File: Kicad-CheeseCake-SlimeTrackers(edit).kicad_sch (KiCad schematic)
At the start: 24 parts, among them J2 USB_C-16p, Q1 UMH3N, SW1 SW_SPDT, U2 TP4057, U3 CH340K

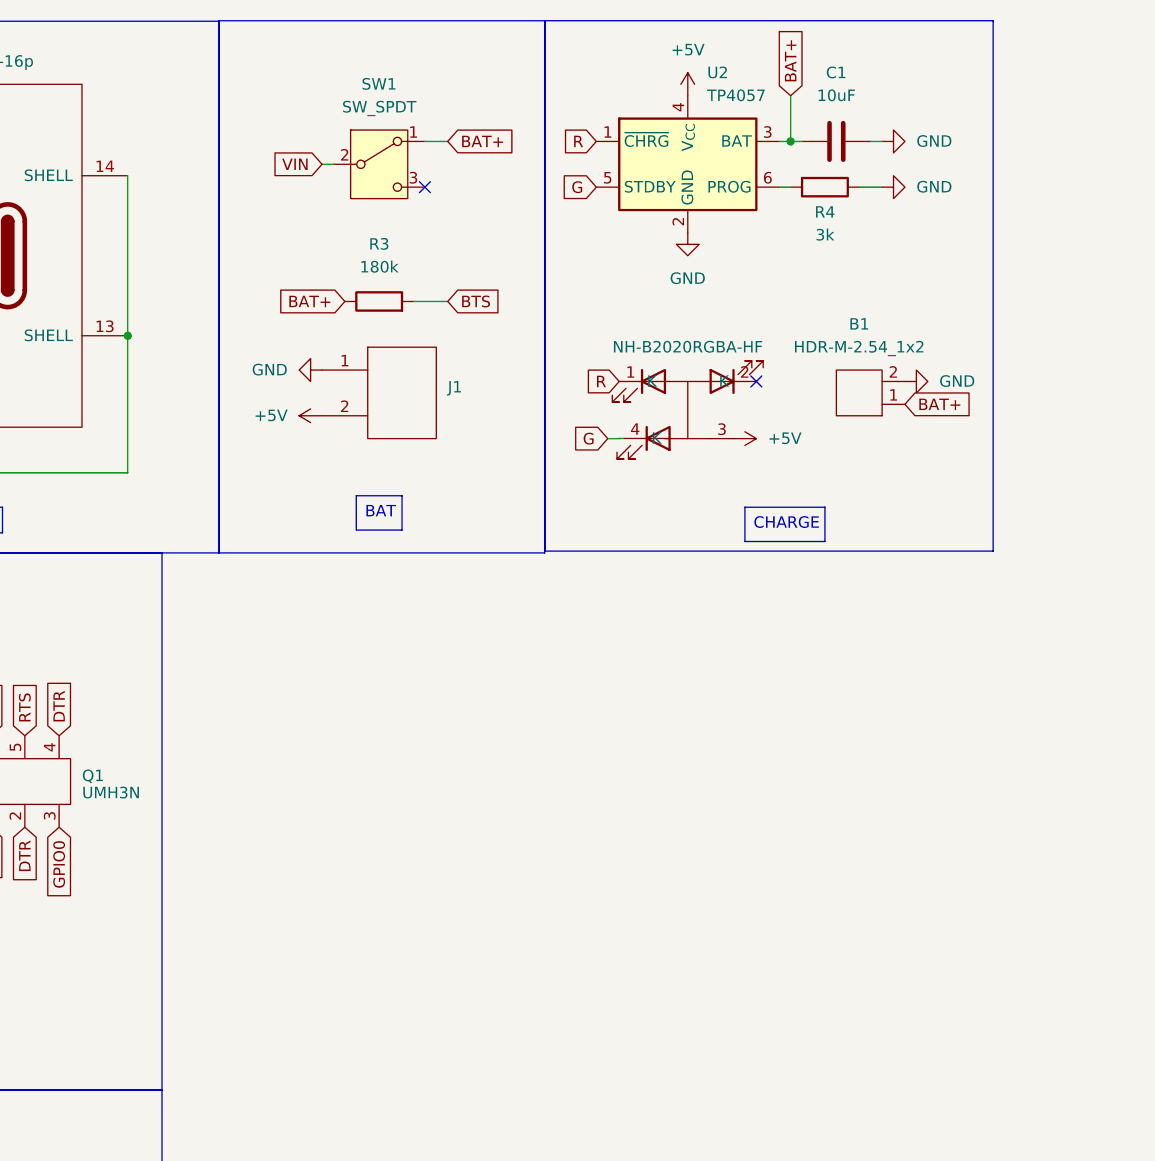
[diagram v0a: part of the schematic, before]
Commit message: updt
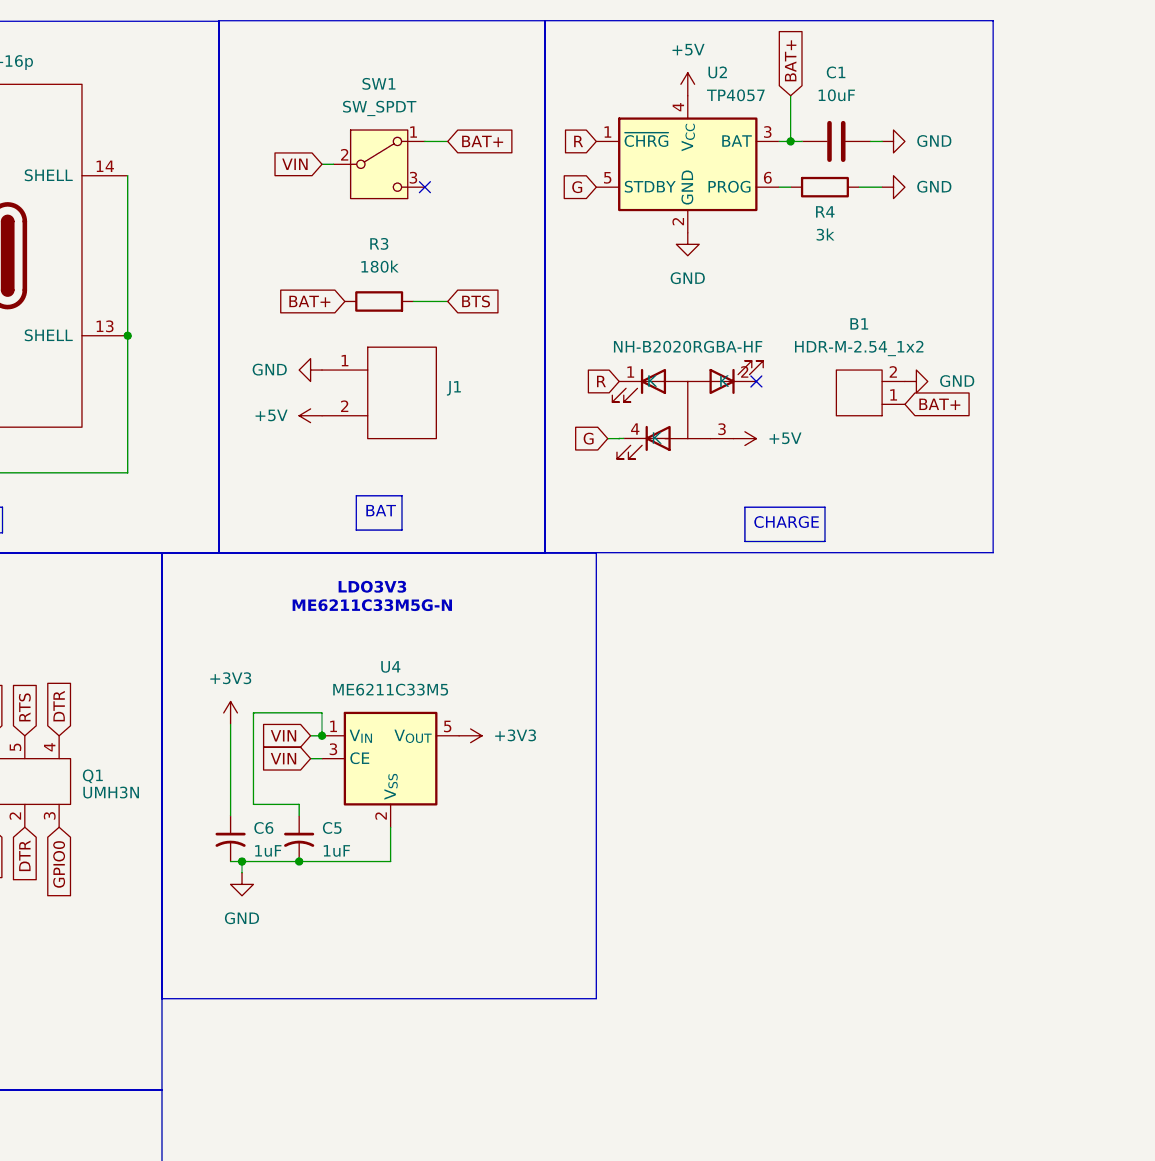
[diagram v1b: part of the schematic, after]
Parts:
- added C5, C6: 1uF, symbol Device:C_Small_US
- added U4: ME6211C33M5, Package_TO_SOT_SMD:SOT-23-5, symbol Regulator_Linear:ME6211C33M5
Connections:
- net +3V3: now also C6.1, U4.5 (V_{OUT})
- net GND: now also C5.2, C6.2, U4.2 (V_{SS})
- net VIN: now also C5.1, U4.1 (V_{IN}), U4.3 (CE)
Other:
- note added: "LDO3V3 ME6211C33M5G-N"

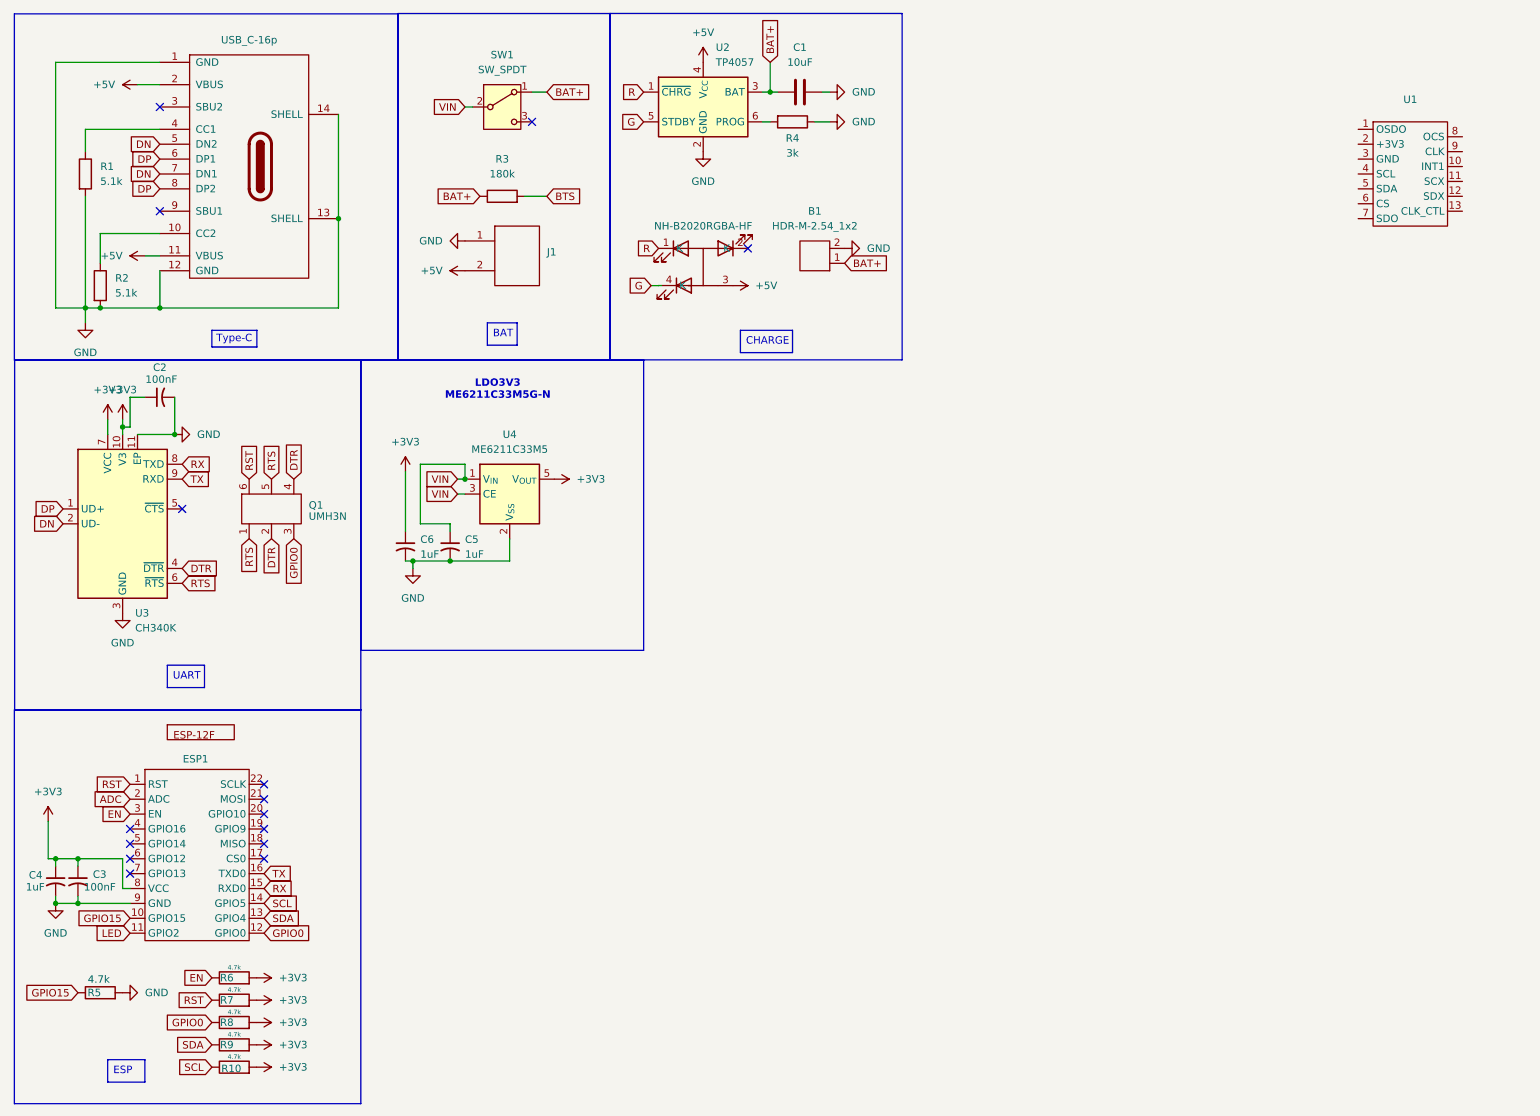
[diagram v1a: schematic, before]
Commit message: updt
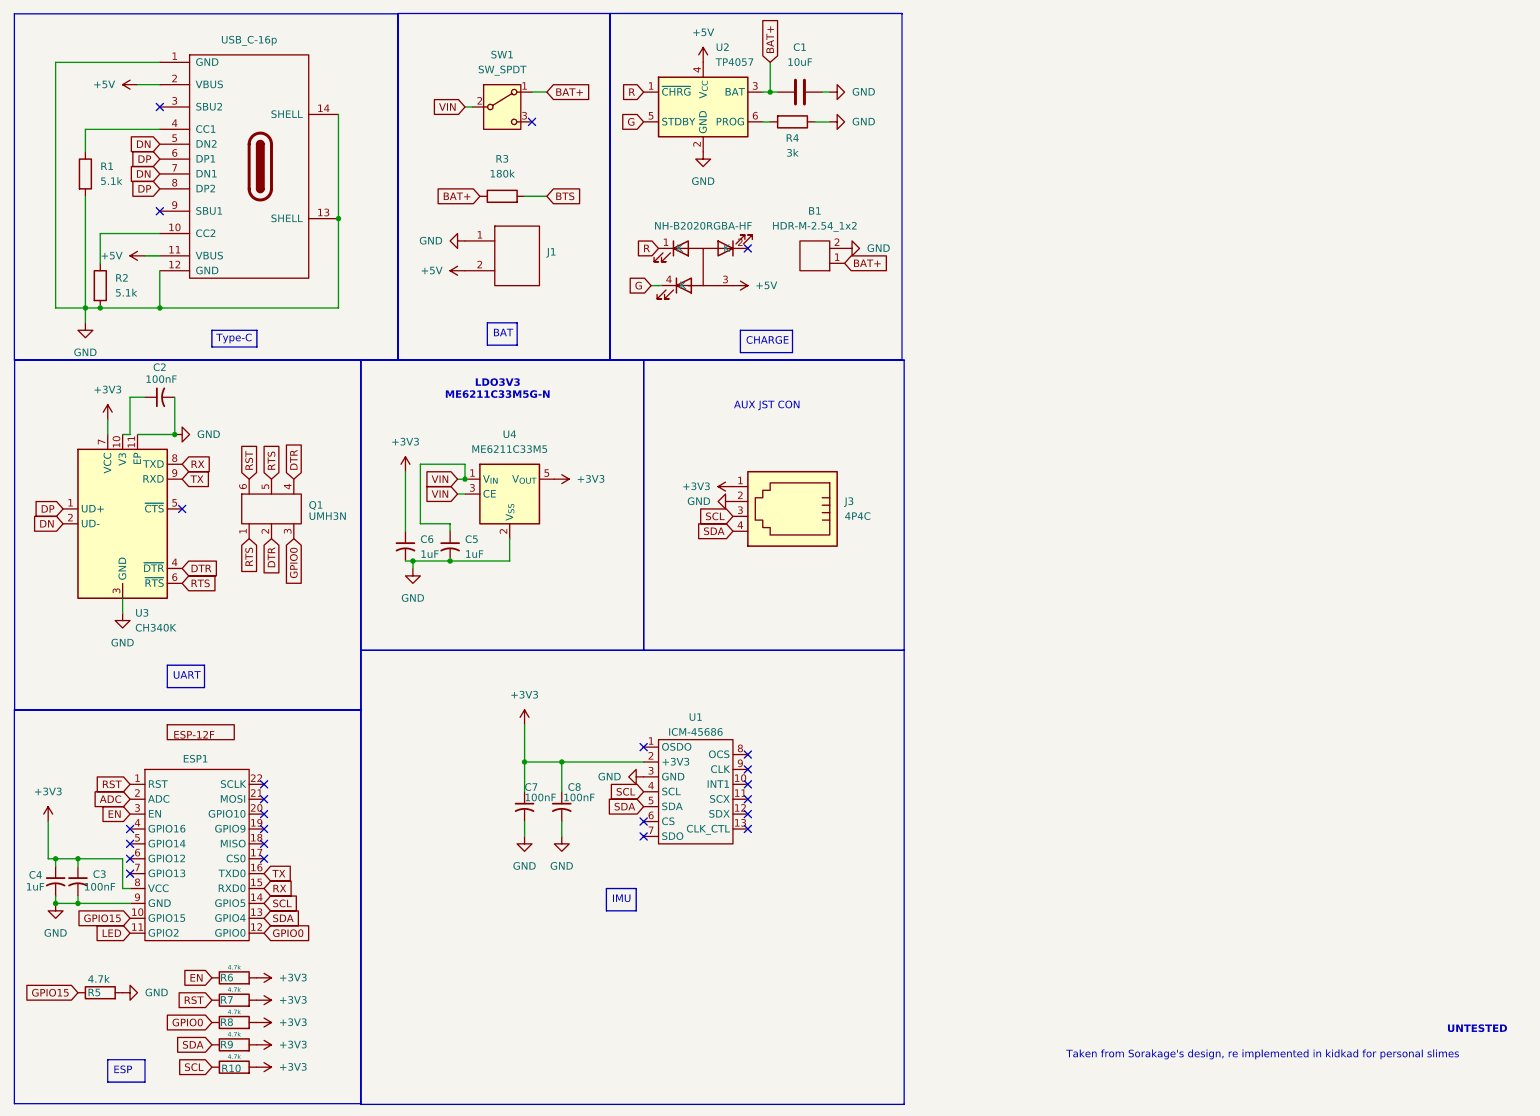
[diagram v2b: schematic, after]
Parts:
- added C7, C8: 100nF, symbol Device:C_Small_US
- added J3: 4P4C, symbol Connector:4P4C
- U1: value ~ -> ICM-45686
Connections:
- net +3V3: now also U1.2 (+3V3), C7.1, C8.1, J3.1; no longer C2.1, U3.10 (V3)
- net GND: now also U1.3 (GND), C7.2, C8.2, J3.2
- net SCL: now also U1.4 (SCL), J3.3
- net SDA: now also U1.5 (SDA), J3.4
- new net: C2.1, U3.10 (V3)
- no-connect marks 15 -> 24
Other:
- note added: "AUX JST CON"
- note added: "Taken from Sorakage's design, re implemented in kidkad for personal slimes"
- note added: "UNTESTED"
- moved on the sheet: U1, U3

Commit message: inital footprint assignment
erc tests passed
some potential issues regarding +3v3 flag - cleared tests for now

some footprints could be wrong and are placeholder
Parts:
- B1, J1: footprint (none) -> Connector_PinHeader_2.54mm:PinHeader_1x02_P2.54mm_Horizontal
- C1, C2, C3, C4, C5, C6, C7, C8: footprint (none) -> Capacitor_SMD:C_0603_1608Metric
- ESP1: footprint (none) -> SlimeFootprints:ESP12F-Devkit-V3
- J2: footprint (none) -> Connector_USB:USB_C_Receptacle_HCTL_HC-TYPE-C-16P-01A
- J3: footprint (none) -> Connector_Hirose:Hirose_DF13C_CL535-0405-0-51_1x05-1MP_P1.25mm_Vertical
- L1: footprint (none) -> LED_SMD:LED_RGB_Cree-PLCC-6_6x5mm_P2.1mm
- Q1: footprint (none) -> Package_TO_SOT_SMD:SOT-363_SC-70-6
- R1, R10, R2, R3, R4, R5, R6, R7, R8, R9: footprint (none) -> Resistor_SMD:R_0603_1608Metric
- SW1: footprint (none) -> SlimeFootprints:SW_SSSS811101
- U1: footprint (none) -> Package_LGA:Bosch_LGA-14_3x2.5mm_P0.5mm
- U3: footprint (none) -> Package_SO:SOIC-10_3.9x4.9mm_P1mm
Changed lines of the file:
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@@
 			)
 		)
-		(property "Footprint" ""
+		(property "Footprint" "Resistor_SMD:R_0603_1608Metric"
 			(at 49.53 185.928 90)
 			(effects
@@
 			)
 		)
-		(property "Footprint" ""
+		(property "Footprint" "Resistor_SMD:R_0603_1608Metric"
 			(at 49.53 182.118 90)
 			(effects
@@
 			)
 		)
-		(property "Footprint" ""
+		(property "Footprint" "Resistor_SMD:R_0603_1608Metric"
 			(at 22.352 39.37 90)
 			(effects
@@
 			)
 		)
-		(property "Footprint" ""
+		(property "Footprint" "Package_LGA:Bosch_LGA-14_3x2.5mm_P0.5mm"
 			(at 128.27 144.78 0)
 			(effects
@@
 			)
 		)
-		(property "Footprint" ""
+		(property "Footprint" "Connector_Hirose:Hirose_DF13C_CL535-0405-0-51_1x05-1MP_P1.25mm_Vertical"
 			(at 144.78 96.52 90)
 			(effects
@@
 			)
 		)
-		(property "Footprint" ""
+		(property "Footprint" "Capacitor_SMD:C_0603_1608Metric"
 			(at 19.05 160.02 0)
 			(effects
@@
 			)
 		)
-		(property "Footprint" ""
+		(property "Footprint" "Capacitor_SMD:C_0603_1608Metric"
 			(at 86.36 102.87 0)
 			(effects
@@
 			)
 		)
-		(property "Footprint" ""
+		(property "Footprint" "Capacitor_SMD:C_0603_1608Metric"
 			(at 78.74 102.87 0)
 			(effects
@@
 			)
 		)
-		(property "Footprint" ""
+		(property "Footprint" "SlimeFootprints:ESP12F-Devkit-V3"
 			(at 43.18 156.21 0)
 			(effects
@@
 			)
 		)
-		(property "Footprint" ""
+		(property "Footprint" "Capacitor_SMD:C_0603_1608Metric"
 			(at 99.06 147.32 0)
 			(effects
@@
 			)
 		)
-		(property "Footprint" ""
+		(property "Footprint" "LED_SMD:LED_RGB_Cree-PLCC-6_6x5mm_P2.1mm"
 			(at 130.81 54.61 0)
 			(effects
@@
 			)
 		)
-		(property "Footprint" ""
+		(property "Footprint" "Connector_PinHeader_2.54mm:PinHeader_1x02_P2.54mm_Horizontal"
 			(at 148.59 53.34 0)
 			(effects
@@
 			)
 		)
-		(property "Footprint" ""
+		(property "Footprint" "Resistor_SMD:R_0603_1608Metric"
 			(at 24.892 58.42 90)
 			(effects
@@
 			)
 		)
-		(property "Footprint" ""
+		(property "Footprint" "Capacitor_SMD:C_0603_1608Metric"
 			(at 36.83 77.47 0)
 			(effects
@@
 			)
 		)
-		(property "Footprint" ""
+		(property "Footprint" "Package_SO:SOIC-10_3.9x4.9mm_P1mm"
 			(at 31.75 113.03 0)
 			(effects
@@
 			)
 		)
-		(property "Footprint" ""
+		(property "Footprint" "Resistor_SMD:R_0603_1608Metric"
 			(at 95.25 44.958 90)
 			(effects
@@
 			)
 		)
-		(property "Footprint" ""
+		(property "Footprint" "Resistor_SMD:R_0603_1608Metric"
 			(at 26.67 180.848 90)
 			(effects
@@
 			)
 		)
-		(property "Footprint" ""
+		(property "Footprint" "Resistor_SMD:R_0603_1608Metric"
 			(at 144.78 28.702 90)
 			(effects
@@
 			)
 		)
-		(property "Footprint" ""
+		(property "Footprint" "Resistor_SMD:R_0603_1608Metric"
 			(at 49.53 193.548 90)
 			(effects
@@
 			)
 		)
-		(property "Footprint" ""
+		(property "Footprint" "Capacitor_SMD:C_0603_1608Metric"
 			(at 105.41 147.32 0)
 			(effects
@@
 			)
 		)
-		(property "Footprint" ""
+		(property "Footprint" "Connector_PinHeader_2.54mm:PinHeader_1x02_P2.54mm_Horizontal"
 			(at 97.79 53.34 0)
 			(effects
@@
 			)
 		)
-		(property "Footprint" ""
+		(property "Footprint" "Capacitor_SMD:C_0603_1608Metric"
 			(at 149.86 24.4348 0)
 			(effects
@@
 			)
 		)
-		(property "Footprint" ""
+		(property "Footprint" "SlimeFootprints:SW_SSSS811101"
 			(at 95.25 27.94 0)
 			(effects
@@
 			)
 		)
-		(property "Footprint" ""
+		(property "Footprint" "Package_TO_SOT_SMD:SOT-363_SC-70-6"
 			(at 55.88 96.52 0)
 			(effects
@@
 			)
 		)
-		(property "Footprint" ""
+		(property "Footprint" "Resistor_SMD:R_0603_1608Metric"
 			(at 49.53 189.738 90)
 			(effects
@@
 			)
 		)
-		(property "Footprint" ""
+		(property "Footprint" "Connector_USB:USB_C_Receptacle_HCTL_HC-TYPE-C-16P-01A"
 			(at 55.88 39.37 0)
 			(effects
@@
 			)
 		)
-		(property "Footprint" ""
+		(property "Footprint" "Resistor_SMD:R_0603_1608Metric"
 			(at 49.53 178.308 90)
 			(effects
@@
 			)
 		)
-		(property "Footprint" ""
+		(property "Footprint" "Capacitor_SMD:C_0603_1608Metric"
 			(at 22.86 160.02 0)
 			(effects
